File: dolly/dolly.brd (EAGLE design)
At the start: 96.5 x 119.4 mm, 31 parts, among them U1 ATTINY85-20P

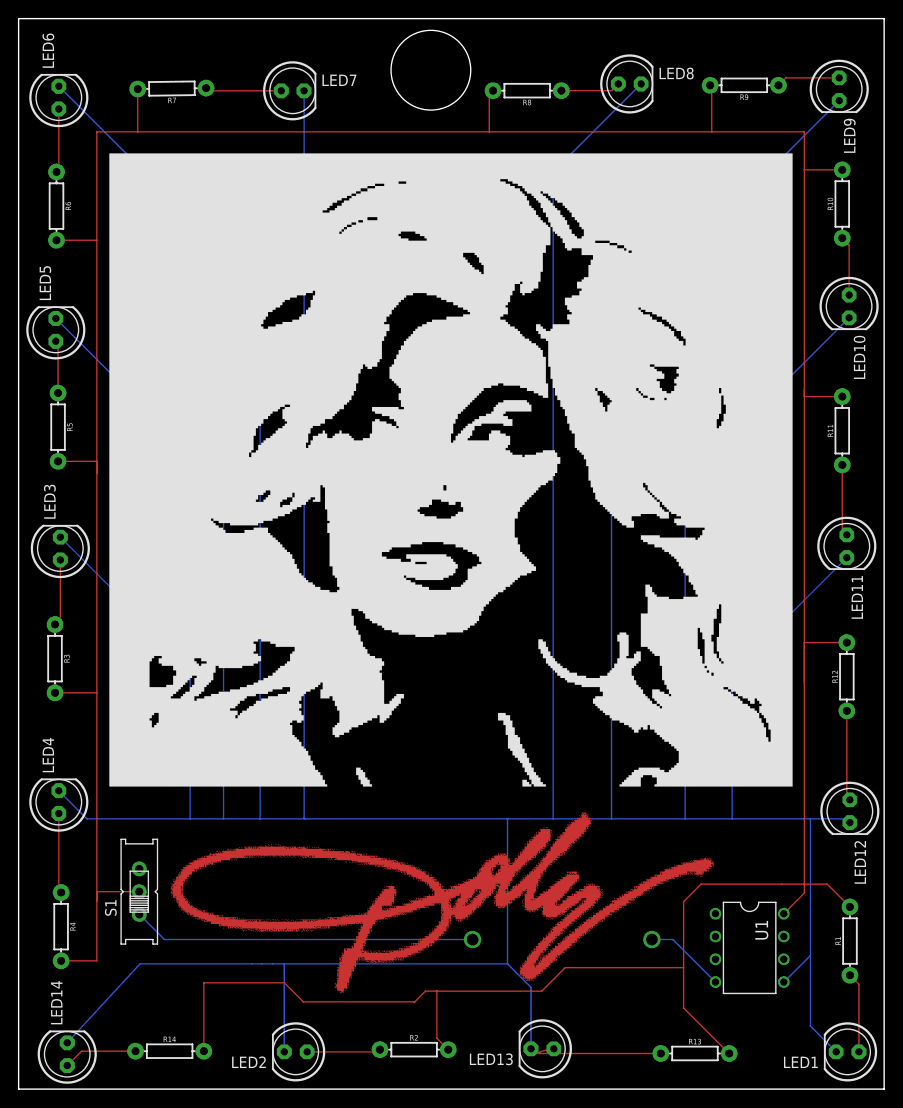
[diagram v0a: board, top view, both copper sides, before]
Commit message: dolly badge
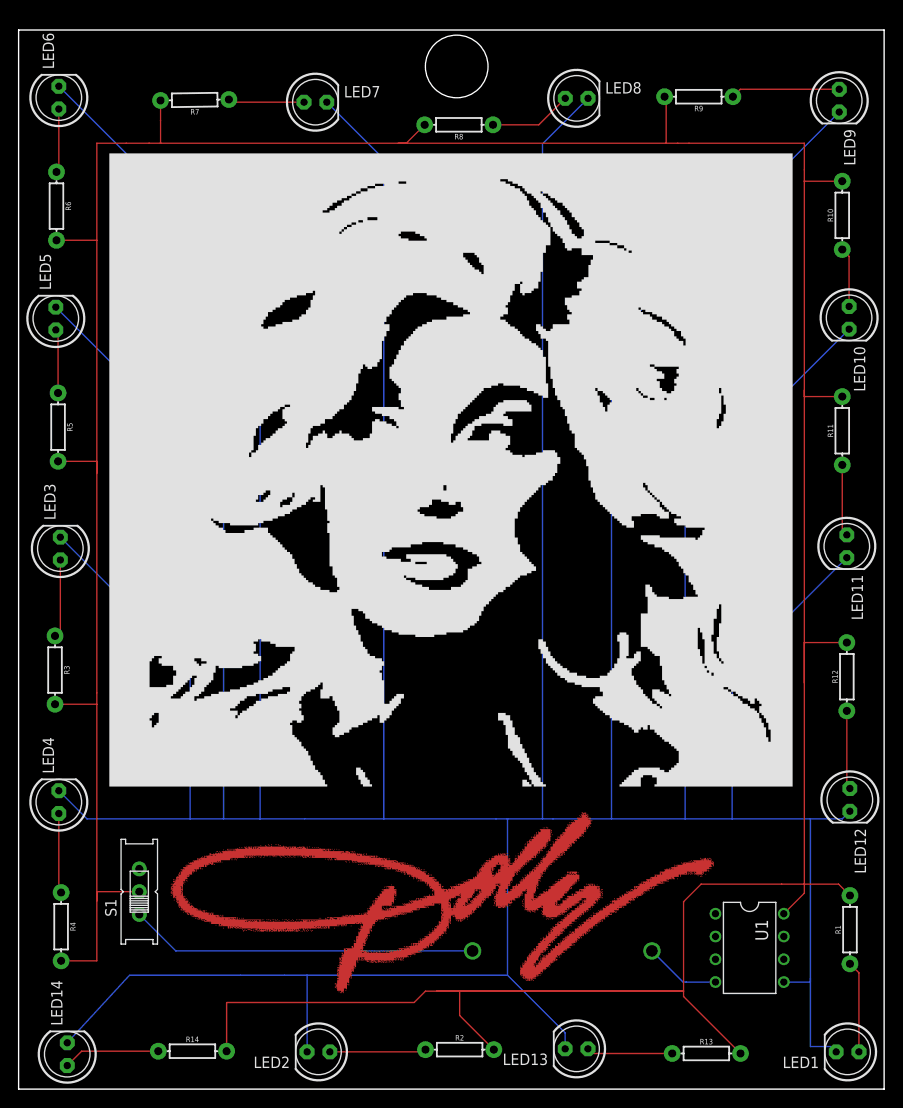
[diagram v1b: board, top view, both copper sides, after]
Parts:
- moved R8 8.52 mm to (38.9, 98.6)
- moved LED8 6.13 mm to (52.1, 101.6)
- moved R9 5.24 mm to (65.7, 101.8)
- moved R2 5.08 mm to (39.0, -4.49)
- moved LED13 3.81 mm to (52.1, -4.40)
- moved R7 2.84 mm to (9.48, 101.4)
- moved LED7 2.84 mm to (22.9, 101.2)
- moved R14 2.54 mm to (9.22, -4.66)
- moved LED2 2.54 mm to (23.3, -4.74)
- moved LED10 1.27 mm to (82.5, 77.1)
- moved LED9 1.27 mm to (81.4, 101.3)
- moved R10 1.27 mm to (81.7, 88.5)
- moved R3 1.27 mm to (-6.10, 37.8)
- moved R1 1.27 mm to (82.5, 8.89)
- moved BT1 1.27 mm to (52.3, 6.52)
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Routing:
- net N$6: track 427.6 -> 448.2 mm
- net N$16: track 16.3 -> 9.61 mm
- net N$12: track 7.12 -> 12.2 mm
- net N$4: track 758.2 -> 755.2 mm
- net N$11: track 6.66 -> 9.28 mm
- net N$17: track 8.28 -> 10.8 mm
- net N$18: track 8.23 -> 10.8 mm
- net N$8: track 5.87 -> 7.14 mm
- net N$3: track 7.80 -> 9.07 mm
- net N$15: track 10.3 -> 8.98 mm
- net N$1: track 8.96 -> 10.2 mm
- net N$5: track 9.05 -> 8.52 mm
- net N$2: track 38.3 -> 38.9 mm
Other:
- board size 96.5 x 119.4 mm -> 96.5 x 118.1 mm
